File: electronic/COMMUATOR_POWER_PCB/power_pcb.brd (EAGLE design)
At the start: 92 x 30.5 mm, 9 parts, among them IC1 L293D, K1 CB1A-P-12V, K2 CB1A-P-12V

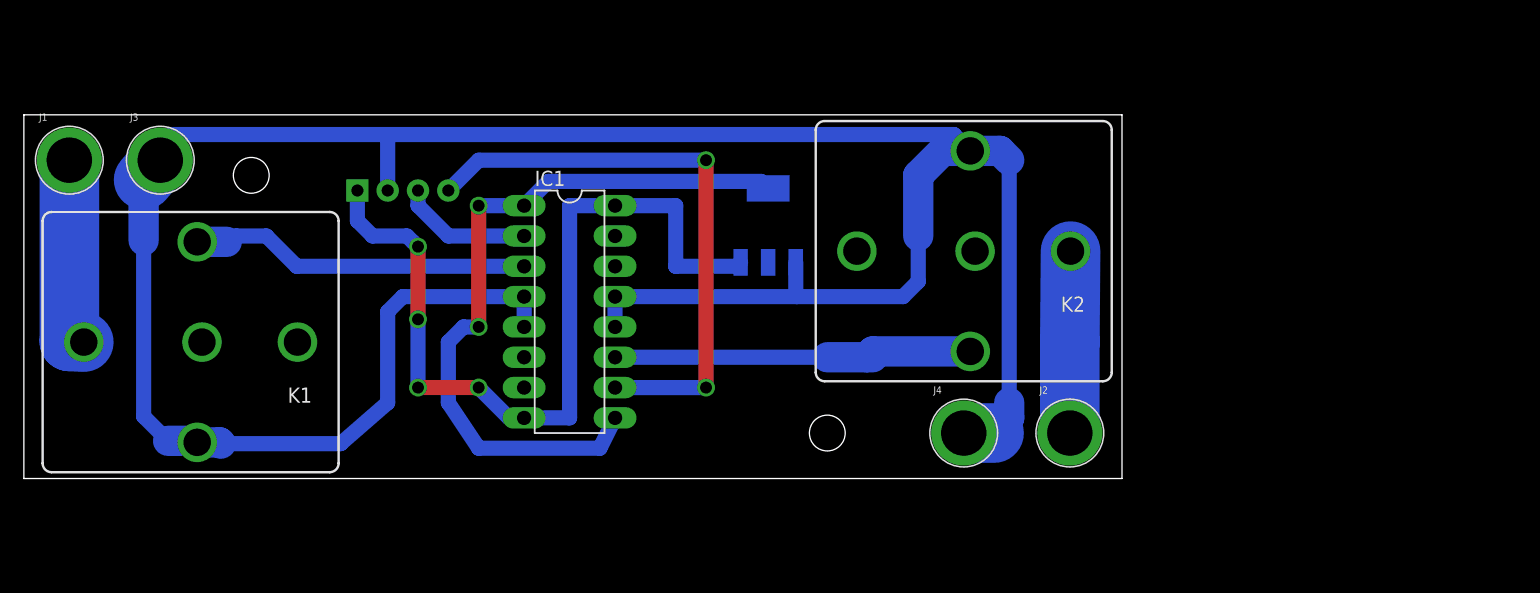
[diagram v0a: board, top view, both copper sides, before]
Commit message: change power pcb
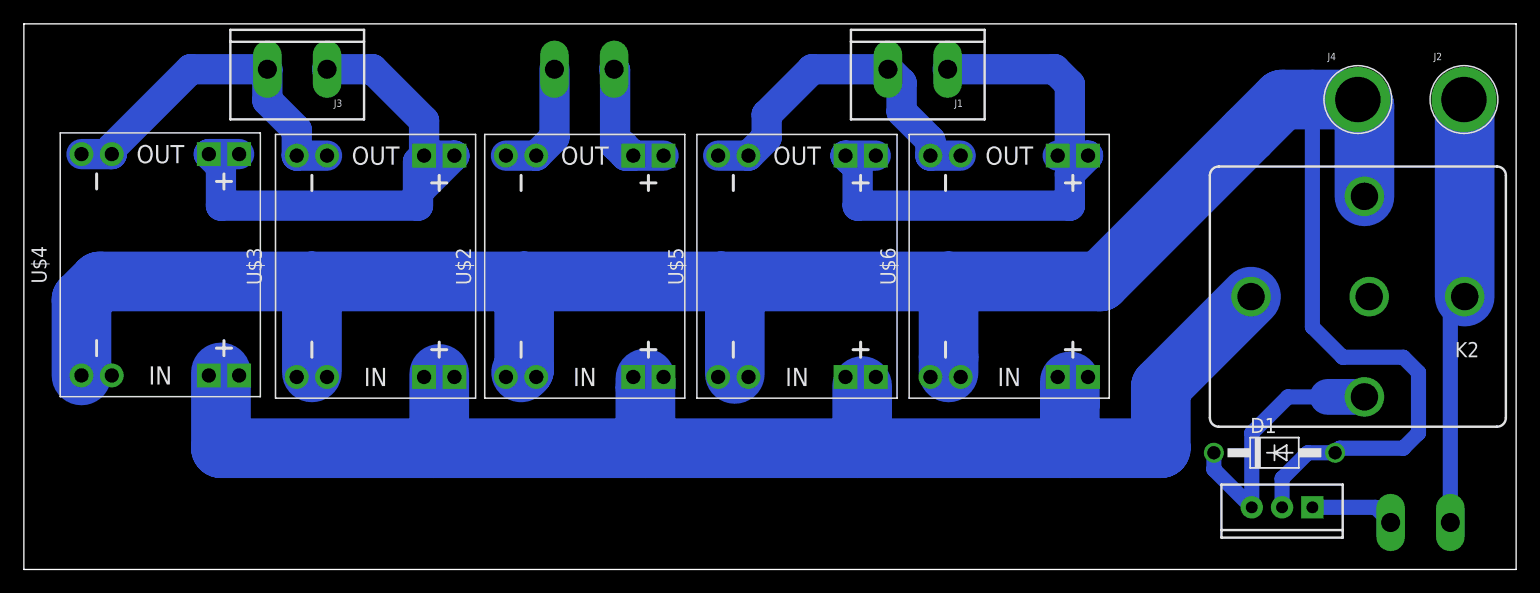
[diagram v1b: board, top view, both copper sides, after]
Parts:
- removed IC1: L293D, st-microelectronics:DIL16
- removed K1: CB1A-P-12V, relay:CB1
- removed U1: (no value), SparkFun-IC-Power:SOT223
- added D1: 1N4004, diode:DO41-10
- added J6: (no value), SparkFun-Connectors:SCREWTERMINAL-5MM-2
- added U$2: 12v, diy-modules:DC-DC-STEP-DOWN-MP1584
- added U$3: usb2, diy-modules:DC-DC-STEP-DOWN-MP1584
- added U$4: USb1, diy-modules:DC-DC-STEP-DOWN-MP1584
- added U$5: Jet2, diy-modules:DC-DC-STEP-DOWN-MP1584
- added U$6: Jet1, diy-modules:DC-DC-STEP-DOWN-MP1584
- added U2: (no value), SparkFun-IC-Power:TO220-IGO
- J1, J3: device SparkFun-Connectors:BANANA_CONN -> SparkFun-Connectors:SCREWTERMINAL-5MM-2
- J5: device SparkFun-Connectors:MOLEX-1X4 -> SparkFun-Connectors:SCREWTERMINAL-5MM-2
- moved J1 74.0 mm to (82.5, 34.3), turned to 180 degrees
- moved J2 43.3 mm to (125.7, 31.8)
- moved J4 43.3 mm to (116.8, 31.8)
- moved K2 33.2 mm to (116.8, 15.2)
- moved J5 19.4 mm to (49.5, 34.3)
- moved J3 15.9 mm to (30.5, 34.3), turned to 180 degrees
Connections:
- removed net +12V: IC1.16, IC1.8, J5.1, U1.3
- removed net +3V3: IC1.1, IC1.9, U1.2, U1.4
- removed net N$1: J1.P$1, K1.30
- removed net REL1: IC1.3, K1.85
- removed net REL2: IC1.11, K2.86
- removed net RELIN1: IC1.2, J5.3
- removed net RELIN2: IC1.10, J5.4
- new net N$11: D1.C, K2.86, U2.OUT
- new net N$13: J6.2, U2.IN
- new net N$4: J1.1, U$5.OUT+.1, U$5.OUT+.2, U$6.OUT+.1, U$6.OUT+.2
- new net N$5: J1.2, U$5.OUT-.1, U$5.OUT-.2, U$6.OUT-.1, U$6.OUT-.2
- new net N$6: J3.2, U$3.OUT-.1, U$3.OUT-.2, U$4.OUT-.1, U$4.OUT-.2
- new net N$7: J3.1, U$3.OUT+.1, U$3.OUT+.2, U$4.OUT+.1, U$4.OUT+.2
- new net N$8: J5.1, U$2.OUT-.1, U$2.OUT-.2
- new net N$9: J5.2, U$2.OUT+.1, U$2.OUT+.2
- net GND: now also D1.A, U$2.IN-.1, U$2.IN-.2, U$3.IN-.1, U$3.IN-.2, U$4.IN-.1, U$4.IN-.2, U$5.IN-.1, U$5.IN-.2, U$6.IN-.1, U$6.IN-.2, U2.GND; no longer IC1.12, IC1.13, IC1.4, IC1.5, J3.P$1, J5.2, K1.86, U1.1
- net N$2: now also J6.1
- net V+: now also U$2.IN+.1, U$2.IN+.2, U$3.IN+.1, U$3.IN+.2, U$4.IN+.1, U$4.IN+.2, U$5.IN+.1, U$5.IN+.2, U$6.IN+.1, U$6.IN+.2; no longer K1.87
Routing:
- net V+: track 0.00 -> 143.9 mm
- net +12V: track 71.4 -> 0.00 mm, vias 4 -> 0
- net +3V3: track 61.2 -> 0.00 mm, vias 2 -> 0
- net N$4: track 0.00 -> 49.4 mm
- net RELIN2: track 49.3 -> 0.00 mm, vias 2 -> 0
- net N$7: track 0.00 -> 47.8 mm
- net REL2: track 33.8 -> 0.00 mm
- net N$6: track 0.00 -> 29.6 mm
- net N$5: track 0.00 -> 29.6 mm
- net REL1: track 28.8 -> 0.00 mm
- net N$11: track 0.00 -> 22.8 mm
- net N$2: track 15.2 -> 36.0 mm
- net N$1: track 16.4 -> 0.00 mm
- net GND: track 217.7 -> 230.7 mm
- net N$9: track 0.00 -> 12.7 mm
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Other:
- board size 92 x 30.5 mm -> 125 x 45.7 mm
